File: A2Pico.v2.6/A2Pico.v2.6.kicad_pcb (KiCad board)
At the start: 2 copper layers, 65.5 x 69.4 mm, 87 parts, among them J1 PinHeader_1x03_P2.54mm_Vertic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, J2 PinHeader_1x04_P2.54mm_Horizo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, T1 TO-92L_Inline_Wide, U1 Pico / PicoW, U2 74LVC245, U3 74LVC245, U4 74LVC245, U5 74F11

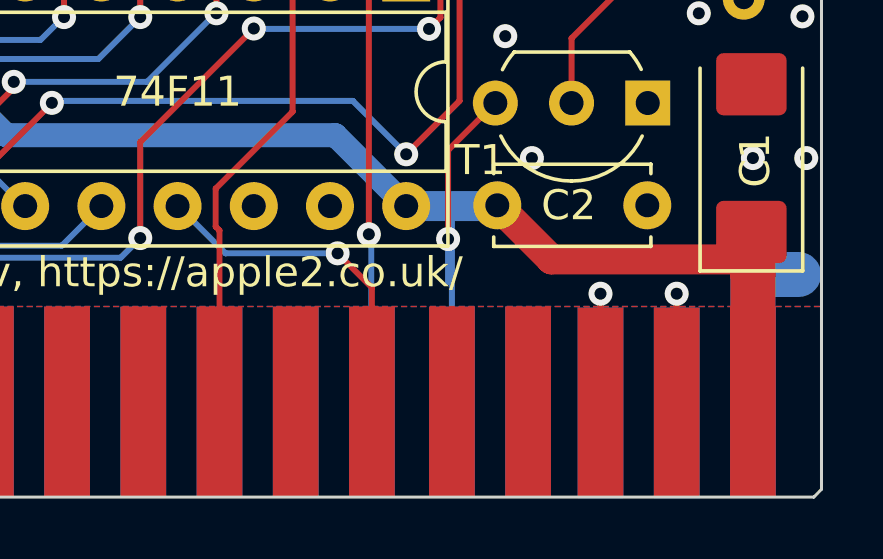
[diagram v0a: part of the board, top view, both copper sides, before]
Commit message: Add files via upload
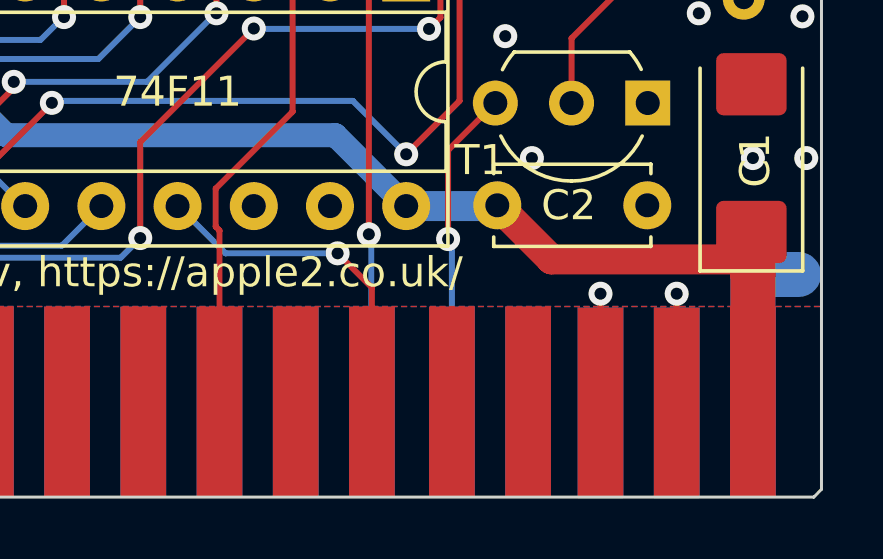
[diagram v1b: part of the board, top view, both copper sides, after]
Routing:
- net IRQ: track 13.1 -> 11.0 mm
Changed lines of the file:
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@@
 		(tags "TO-92L Inline Wide transistor")
 		(property "Reference" "T1"
-			(at 5.588 -1.905 360)
+			(at 5.588 -1.905 0)
 			(layer "F.SilkS")
 			(effects
@@
 		)
 		(property "Value" "TO-92L_Inline_Wide"
-			(at 2.54 2.79 360)
+			(at 2.54 2.79 0)
 			(layer "F.Fab")
 			(hide yes)
@@
 		)
 		(property "Footprint" ""
-			(at 0 0 360)
+			(at 0 0 0)
 			(layer "F.Fab")
 			(hide yes)
@@
 		)
 		(property "Datasheet" ""
-			(at 0 0 360)
+			(at 0 0 0)
 			(layer "F.Fab")
 			(hide yes)
@@
 		)
 		(property "Description" ""
-			(at 0 0 360)
+			(at 0 0 0)
 			(layer "F.Fab")
 			(hide yes)
@@
 		)
 		(fp_text user "${REFERENCE}"
-			(at 2.54 0 360)
+			(at 2.54 0 0)
 			(layer "F.Fab")
 			(hide yes)
@@
 	)
 	(segment
-		(start 157.099 113.7791)
-		(end 157.099 115.2144)
+		(start 157.226 119.558658)
+		(end 157.226 113.9061)
 		(width 0.2)
 		(layer "B.Cu")
@@
 	)
 	(segment
-		(start 157.226 119.558658)
-		(end 157.226 113.062293)
+		(start 157.226 113.9061)
+		(end 157.099 113.7791)
 		(width 0.2)
 		(layer "B.Cu")
